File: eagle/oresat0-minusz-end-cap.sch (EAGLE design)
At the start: 33 parts, among them J1 6-104178-1, U1 LTC4305, U2 MMC5883MA, U3 MMC5883MA

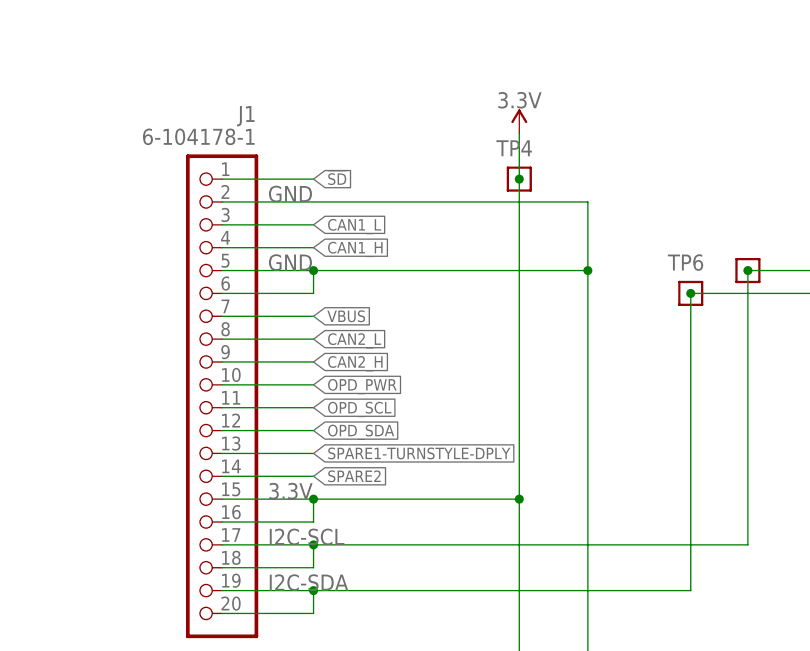
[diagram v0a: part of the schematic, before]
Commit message: v1.0 end caps for OreSat0!
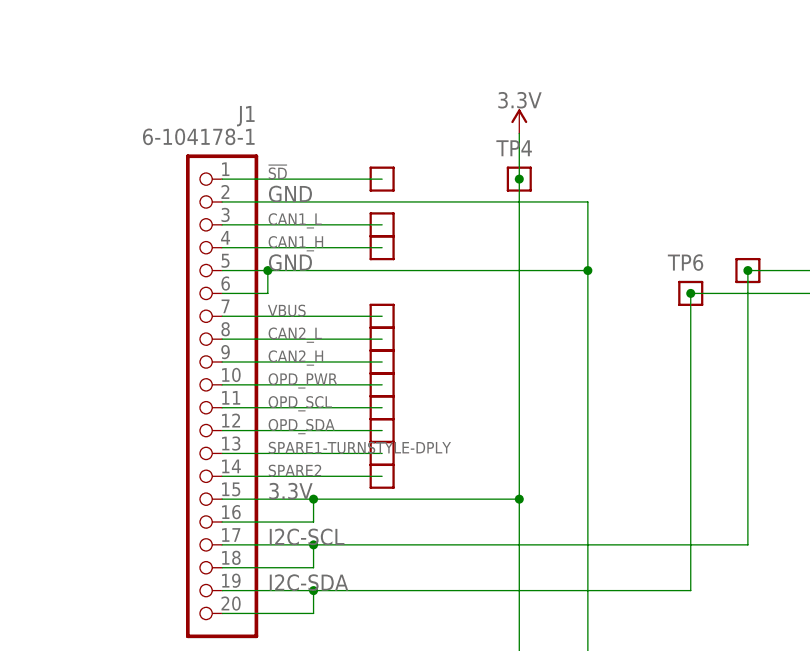
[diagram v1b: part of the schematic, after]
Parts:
- added TP10, TP11, TP12, TP13, TP14, TP15, TP16, TP17, TP18, TP19, TP9: TEST-POINT-LARGE-SQUARE, oresat-misc:TEST-POINT-LARGE-SQUARE
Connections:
- net !SD: now also TP9.1
- net CAN1_H: now also TP11.1
- net CAN1_L: now also TP10.1
- net CAN2_H: now also TP14.1
- net CAN2_L: now also TP13.1
- net OPD_PWR: now also TP15.1
- net OPD_SCL: now also TP16.1
- net OPD_SDA: now also TP17.1
- net SPARE1-TURNSTYLE-DPLY: now also TP18.1
- net SPARE2: now also TP19.1
- net VBUS: now also TP12.1
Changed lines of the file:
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@@
 <?xml version="1.0" encoding="utf-8"?>
 <!DOCTYPE eagle SYSTEM "eagle.dtd">
-<eagle version="9.5.1">
+<eagle version="9.6.1">
 <drawing>
 <settings>
@@
 <setting verticaltext="up"/>
 </settings>
-<grid distance="0.05" unitdist="inch" unit="inch" style="lines" multiple="1" display="no" altdistance="0.01" altunitdist="inch" altunit="inch"/>
+<grid distance="0.1" unitdist="inch" unit="inch" style="lines" multiple="1" display="no" altdistance="0.01" altunitdist="inch" altunit="inch"/>
 <layers>
 <layer number="1" name="Top" color="4" fill="1" visible="no" active="no"/>
@@
 </part>
 <part name="J1" library="J-TE-6-104178-1-1.27mm-male-th" deviceset="6-104178-1" device=""/>
+<part name="TP9" library="oresat-misc" deviceset="TEST-POINT-LARGE-SQUARE" device=""/>
+<part name="TP10" library="oresat-misc" deviceset="TEST-POINT-LARGE-SQUARE" device=""/>
+<part name="TP11" library="oresat-misc" deviceset="TEST-POINT-LARGE-SQUARE" device=""/>
+<part name="TP12" library="oresat-misc" deviceset="TEST-POINT-LARGE-SQUARE" device=""/>
+<part name="TP13" library="oresat-misc" deviceset="TEST-POINT-LARGE-SQUARE" device=""/>
+<part name="TP14" library="oresat-misc" deviceset="TEST-POINT-LARGE-SQUARE" device=""/>
+<part name="TP15" library="oresat-misc" deviceset="TEST-POINT-LARGE-SQUARE" device=""/>
+<part name="TP16" library="oresat-misc" deviceset="TEST-POINT-LARGE-SQUARE" device=""/>
+<part name="TP17" library="oresat-misc" deviceset="TEST-POINT-LARGE-SQUARE" device=""/>
+<part name="TP18" library="oresat-misc" deviceset="TEST-POINT-LARGE-SQUARE" device=""/>
+<part name="TP19" library="oresat-misc" deviceset="TEST-POINT-LARGE-SQUARE" device=""/>
 </parts>
 <sheets>
@@
 <attribute name="VALUE" x="82.55" y="168.91" size="1.778" layer="96" rot="MR0"/>
 </instance>
+<instance part="TP9" gate="G$1" x="96.52" y="165.1" smashed="yes">
+<attribute name="NAME" x="99.06" y="165.1" size="1.27" layer="104"/>
+</instance>
+<instance part="TP10" gate="G$1" x="96.52" y="160.02" smashed="yes">
+<attribute name="NAME" x="99.06" y="160.02" size="1.27" layer="104"/>
+</instance>
+<instance part="TP11" gate="G$1" x="96.52" y="157.48" smashed="yes">
+<attribute name="NAME" x="99.06" y="157.48" size="1.27" layer="104"/>
+</instance>
+<instance part="TP12" gate="G$1" x="96.52" y="149.86" smashed="yes">
+<attribute name="NAME" x="99.06" y="149.86" size="1.27" layer="104"/>
+</instance>
+<instance part="TP13" gate="G$1" x="96.52" y="147.32" smashed="yes">
+<attribute name="NAME" x="99.06" y="147.32" size="1.27" layer="104"/>
+</instance>
+<instance part="TP14" gate="G$1" x="96.52" y="144.78" smashed="yes">
+<attribute name="NAME" x="99.06" y="144.78" size="1.27" layer="104"/>
+</instance>
+<instance part="TP15" gate="G$1" x="96.52" y="142.24" smashed="yes">
+<attribute name="NAME" x="99.06" y="142.24" size="1.27" layer="104"/>
+</instance>
+<instance part="TP16" gate="G$1" x="96.52" y="139.7" smashed="yes">
+<attribute name="NAME" x="99.06" y="139.7" size="1.27" layer="104"/>
+</instance>
+<instance part="TP17" gate="G$1" x="96.52" y="137.16" smashed="yes">
+<attribute name="NAME" x="99.06" y="137.16" size="1.27" layer="104"/>
+</instance>
+<instance part="TP18" gate="G$1" x="96.52" y="134.62" smashed="yes">
+<attribute name="NAME" x="99.06" y="134.62" size="1.27" layer="104"/>
+</instance>
+<instance part="TP19" gate="G$1" x="96.52" y="132.08" smashed="yes">
+<attribute name="NAME" x="99.06" y="132.08" size="1.27" layer="104"/>
+</instance>
 </instances>
 <busses>
@@
 <wire x1="78.74" y1="162.56" x2="119.38" y2="162.56" width="0.1524" layer="91"/>
 <pinref part="J1" gate="G$1" pin="5"/>
-<wire x1="78.74" y1="154.94" x2="88.9" y2="154.94" width="0.1524" layer="91"/>
+<wire x1="78.74" y1="154.94" x2="83.82" y2="154.94" width="0.1524" layer="91"/>
 <junction x="119.38" y="154.94"/>
 <pinref part="J1" gate="G$1" pin="6"/>
-<wire x1="88.9" y1="154.94" x2="119.38" y2="154.94" width="0.1524" layer="91"/>
-<wire x1="78.74" y1="152.4" x2="88.9" y2="152.4" width="0.1524" layer="91"/>
-<wire x1="88.9" y1="152.4" x2="88.9" y2="154.94" width="0.1524" layer="91"/>
-<junction x="88.9" y="154.94"/>
+<wire x1="83.82" y1="154.94" x2="119.38" y2="154.94" width="0.1524" layer="91"/>
+<wire x1="78.74" y1="152.4" x2="83.82" y2="152.4" width="0.1524" layer="91"/>
+<wire x1="83.82" y1="152.4" x2="83.82" y2="154.94" width="0.1524" layer="91"/>
+<junction x="83.82" y="154.94"/>
 <label x="83.82" y="162.56" size="1.778" layer="95"/>
 <label x="83.82" y="154.94" size="1.778" layer="95"/>
@@
 <segment>
 <pinref part="J1" gate="G$1" pin="1"/>
-<wire x1="78.74" y1="165.1" x2="88.9" y2="165.1" width="0.1524" layer="91"/>
-<label x="88.9" y="165.1" size="1.27" layer="95" xref="yes"/>
+<label x="83.82" y="165.1" size="1.27" layer="95"/>
+<pinref part="TP9" gate="G$1" pin="1"/>
+<wire x1="78.74" y1="165.1" x2="96.52" y2="165.1" width="0.1524" layer="91"/>
 </segment>
 </net>
@@
 <segment>
 <pinref part="J1" gate="G$1" pin="3"/>
-<wire x1="78.74" y1="160.02" x2="88.9" y2="160.02" width="0.1524" layer="91"/>
-<label x="88.9" y="160.02" size="1.27" layer="95" xref="yes"/>
+<label x="83.82" y="160.02" size="1.27" layer="95"/>
+<pinref part="TP10" gate="G$1" pin="1"/>
+<wire x1="78.74" y1="160.02" x2="96.52" y2="160.02" width="0.1524" layer="91"/>
 </segment>
 </net>
@@
 <segment>
 <pinref part="J1" gate="G$1" pin="4"/>
-<wire x1="78.74" y1="157.48" x2="88.9" y2="157.48" width="0.1524" layer="91"/>
-<label x="88.9" y="157.48" size="1.27" layer="95" xref="yes"/>
+<label x="83.82" y="157.48" size="1.27" layer="95"/>
+<pinref part="TP11" gate="G$1" pin="1"/>
+<wire x1="96.52" y1="157.48" x2="78.74" y2="157.48" width="0.1524" layer="91"/>
 </segment>
 </net>
@@
 <segment>
 <pinref part="J1" gate="G$1" pin="7"/>
-<wire x1="78.74" y1="149.86" x2="88.9" y2="149.86" width="0.1524" layer="91"/>
-<label x="88.9" y="149.86" size="1.27" layer="95" xref="yes"/>
+<label x="83.82" y="149.86" size="1.27" layer="95"/>
+<pinref part="TP12" gate="G$1" pin="1"/>
+<wire x1="78.74" y1="149.86" x2="96.52" y2="149.86" width="0.1524" layer="91"/>
 </segment>
 </net>
@@
 <segment>
 <pinref part="J1" gate="G$1" pin="8"/>
-<wire x1="78.74" y1="147.32" x2="88.9" y2="147.32" width="0.1524" layer="91"/>
-<label x="88.9" y="147.32" size="1.27" layer="95" xref="yes"/>
+<label x="83.82" y="147.32" size="1.27" layer="95"/>
+<pinref part="TP13" gate="G$1" pin="1"/>
+<wire x1="96.52" y1="147.32" x2="78.74" y2="147.32" width="0.1524" layer="91"/>
 </segment>
 </net>
@@
 <segment>
 <pinref part="J1" gate="G$1" pin="9"/>
-<wire x1="78.74" y1="144.78" x2="88.9" y2="144.78" width="0.1524" layer="91"/>
-<label x="88.9" y="144.78" size="1.27" layer="95" xref="yes"/>
+<label x="83.82" y="144.78" size="1.27" layer="95"/>
+<pinref part="TP14" gate="G$1" pin="1"/>
+<wire x1="78.74" y1="144.78" x2="96.52" y2="144.78" width="0.1524" layer="91"/>
 </segment>
 </net>
@@
 <segment>
 <pinref part="J1" gate="G$1" pin="10"/>
-<wire x1="78.74" y1="142.24" x2="88.9" y2="142.24" width="0.1524" layer="91"/>
-<label x="88.9" y="142.24" size="1.27" layer="95" xref="yes"/>
+<label x="83.82" y="142.24" size="1.27" layer="95"/>
+<pinref part="TP15" gate="G$1" pin="1"/>
+<wire x1="96.52" y1="142.24" x2="78.74" y2="142.24" width="0.1524" layer="91"/>
 </segment>
 </net>
@@
 <segment>
 <pinref part="J1" gate="G$1" pin="11"/>
-<wire x1="78.74" y1="139.7" x2="88.9" y2="139.7" width="0.1524" layer="91"/>
-<label x="88.9" y="139.7" size="1.27" layer="95" xref="yes"/>
+<label x="83.82" y="139.7" size="1.27" layer="95"/>
+<pinref part="TP16" gate="G$1" pin="1"/>
+<wire x1="78.74" y1="139.7" x2="96.52" y2="139.7" width="0.1524" layer="91"/>
 </segment>
 </net>
@@
 <segment>
 <pinref part="J1" gate="G$1" pin="12"/>
-<wire x1="78.74" y1="137.16" x2="88.9" y2="137.16" width="0.1524" layer="91"/>
-<label x="88.9" y="137.16" size="1.27" layer="95" xref="yes"/>
+<label x="83.82" y="137.16" size="1.27" layer="95"/>
+<pinref part="TP17" gate="G$1" pin="1"/>
+<wire x1="96.52" y1="137.16" x2="78.74" y2="137.16" width="0.1524" layer="91"/>
 </segment>
 </net>
@@
 <segment>
 <pinref part="J1" gate="G$1" pin="13"/>
-<wire x1="78.74" y1="134.62" x2="88.9" y2="134.62" width="0.1524" layer="91"/>
-<label x="88.9" y="134.62" size="1.27" layer="95" xref="yes"/>
+<label x="83.82" y="134.62" size="1.27" layer="95"/>
+<pinref part="TP18" gate="G$1" pin="1"/>
+<wire x1="78.74" y1="134.62" x2="96.52" y2="134.62" width="0.1524" layer="91"/>
 </segment>
 </net>
@@
 <segment>
 <pinref part="J1" gate="G$1" pin="14"/>
-<wire x1="78.74" y1="132.08" x2="88.9" y2="132.08" width="0.1524" layer="91"/>
-<label x="88.9" y="132.08" size="1.27" layer="95" xref="yes"/>
-</segment>
-</net>
+<label x="83.82" y="132.08" size="1.27" layer="95"/>
+<pinref part="TP19" gate="G$1" pin="1"/>
+<wire x1="96.52" y1="132.08" x2="78.74" y2="132.08" width="0.1524" layer="91"/>
+</segment>
+</net>
